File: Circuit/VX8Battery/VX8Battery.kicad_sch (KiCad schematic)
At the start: 28 parts, among them J1 USBC-Molex-2171780001, J2 VX8BattPins, U1 MP2672A

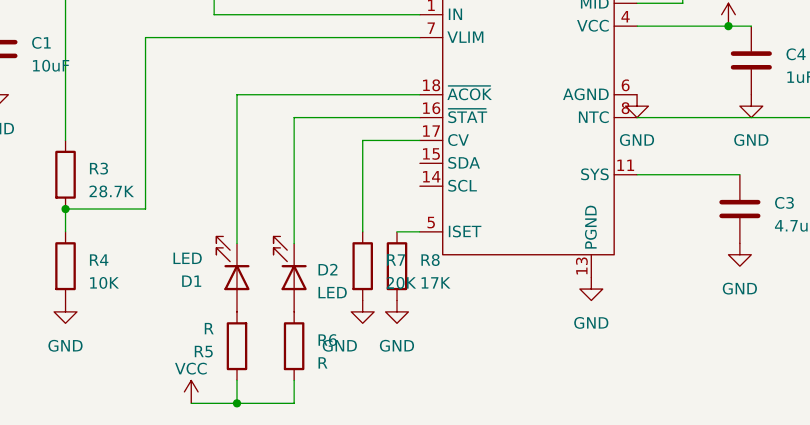
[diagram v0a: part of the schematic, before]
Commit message: Added stl, removed backups
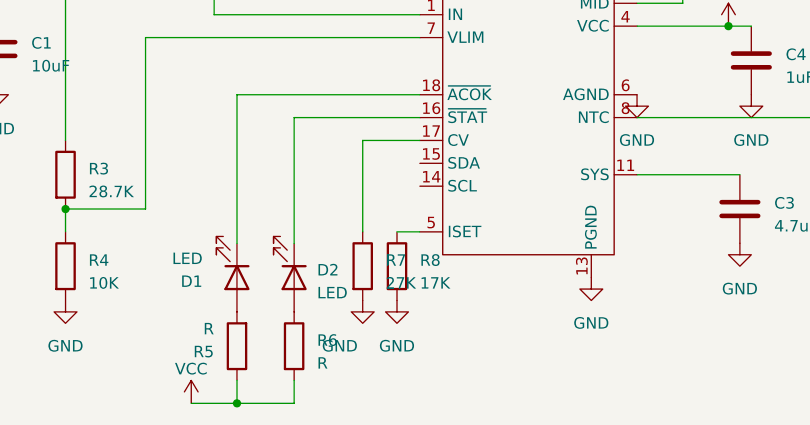
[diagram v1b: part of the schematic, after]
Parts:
- R7: value 20K -> 27K
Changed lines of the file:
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@@
       (effects (font (size 1.27 1.27)) (justify left))
     )
-    (property "Value" "20K" (id 1) (at 113.03 133.9849 0)
+    (property "Value" "27K" (id 1) (at 113.03 133.9849 0)
       (effects (font (size 1.27 1.27)) (justify left))
     )
@@
     )
     (path "/ff1faed0-c978-4f89-b883-3b48c66f37b7"
-      (reference "R7") (unit 1) (value "20K") (footprint "Resistor_SMD:R_0603_1608Metric")
+      (reference "R7") (unit 1) (value "27K") (footprint "Resistor_SMD:R_0603_1608Metric")
     )
     (path "/220e215a-7b41-4034-b105-3f629371f423"
